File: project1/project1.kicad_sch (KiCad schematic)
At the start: 7 parts, among them U1 TJA1050T, U2 MCP2515-xST, U3 STM32G474RBTx

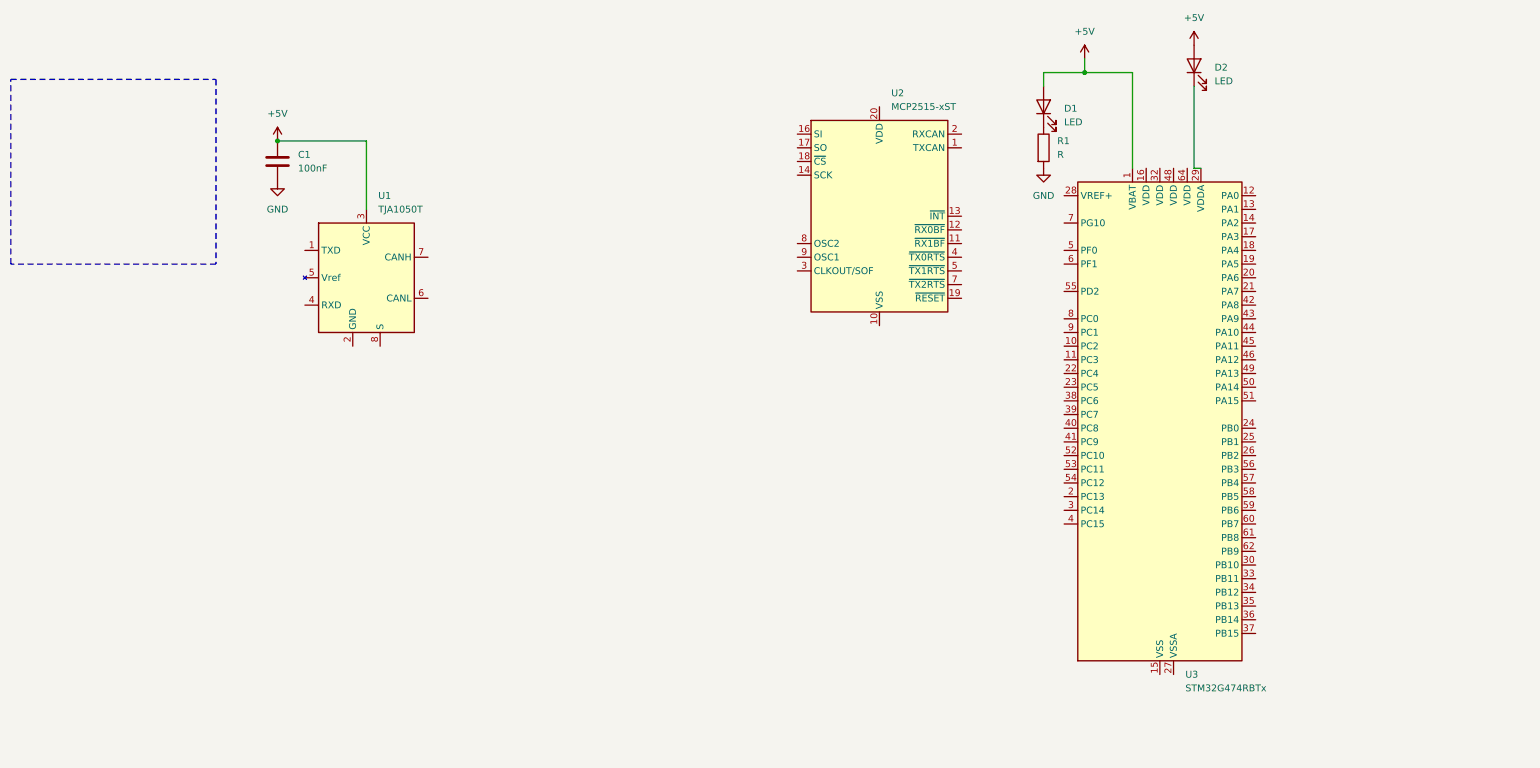
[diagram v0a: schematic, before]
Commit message: avancements sur l'alimentation du STM32
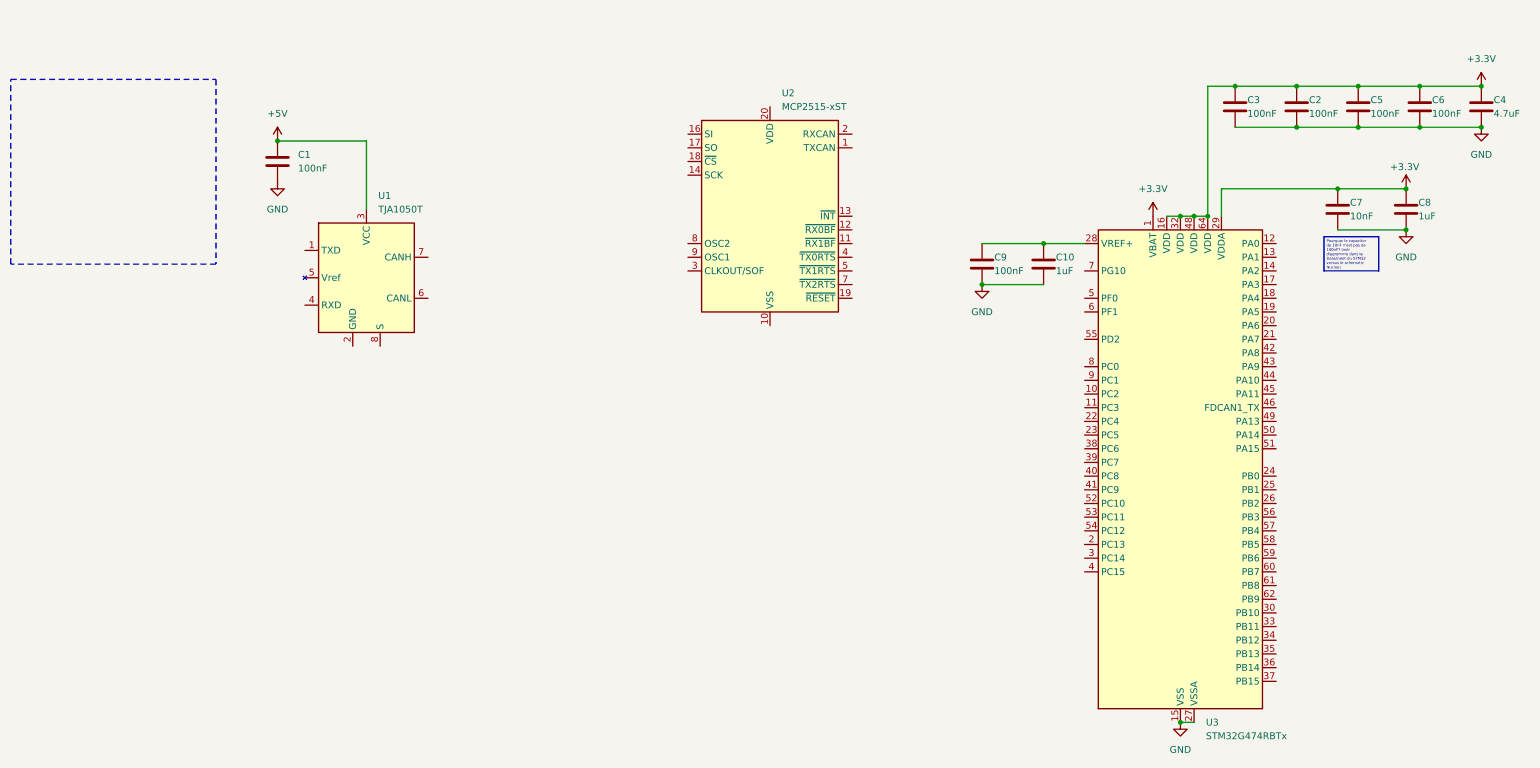
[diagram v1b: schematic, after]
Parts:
- removed D1, D2: LED, symbol Device:LED
- removed R1: R, symbol Device:R
- added C10, C8: 1uF, symbol Device:C
- added C2, C3, C5, C6, C9: 100nF, symbol Device:C
- added C4: 4.7uF, symbol Device:C
- added C7: 10nF, symbol Device:C
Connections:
- net +5V: no longer U3.1 (VBAT)
- net GND: now also U3.15 (VSS), U3.27 (VSSA), U3.31 (VSS), U3.47 (VSS), U3.63 (VSS), C10.2, C2.2, C3.2, C4.2, C5.2, C6.2, C7.2, C8.2, C9.2
- net +3.3V: now reaches U3.16 (VDD)
- net +3.3V: now also U3.1 (VBAT), U3.29 (VDDA), U3.32 (VDD), U3.48 (VDD), U3.64 (VDD), C2.1, C3.1, C4.1, C5.1, C6.1, C7.1, C8.1
- net at U3.28 (VREF+): now also C10.1, C9.1
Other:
- moved on the sheet: U2, U3
